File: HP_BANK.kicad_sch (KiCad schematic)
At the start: 1 part, among them J7 Conn_02x70_Odd_Even

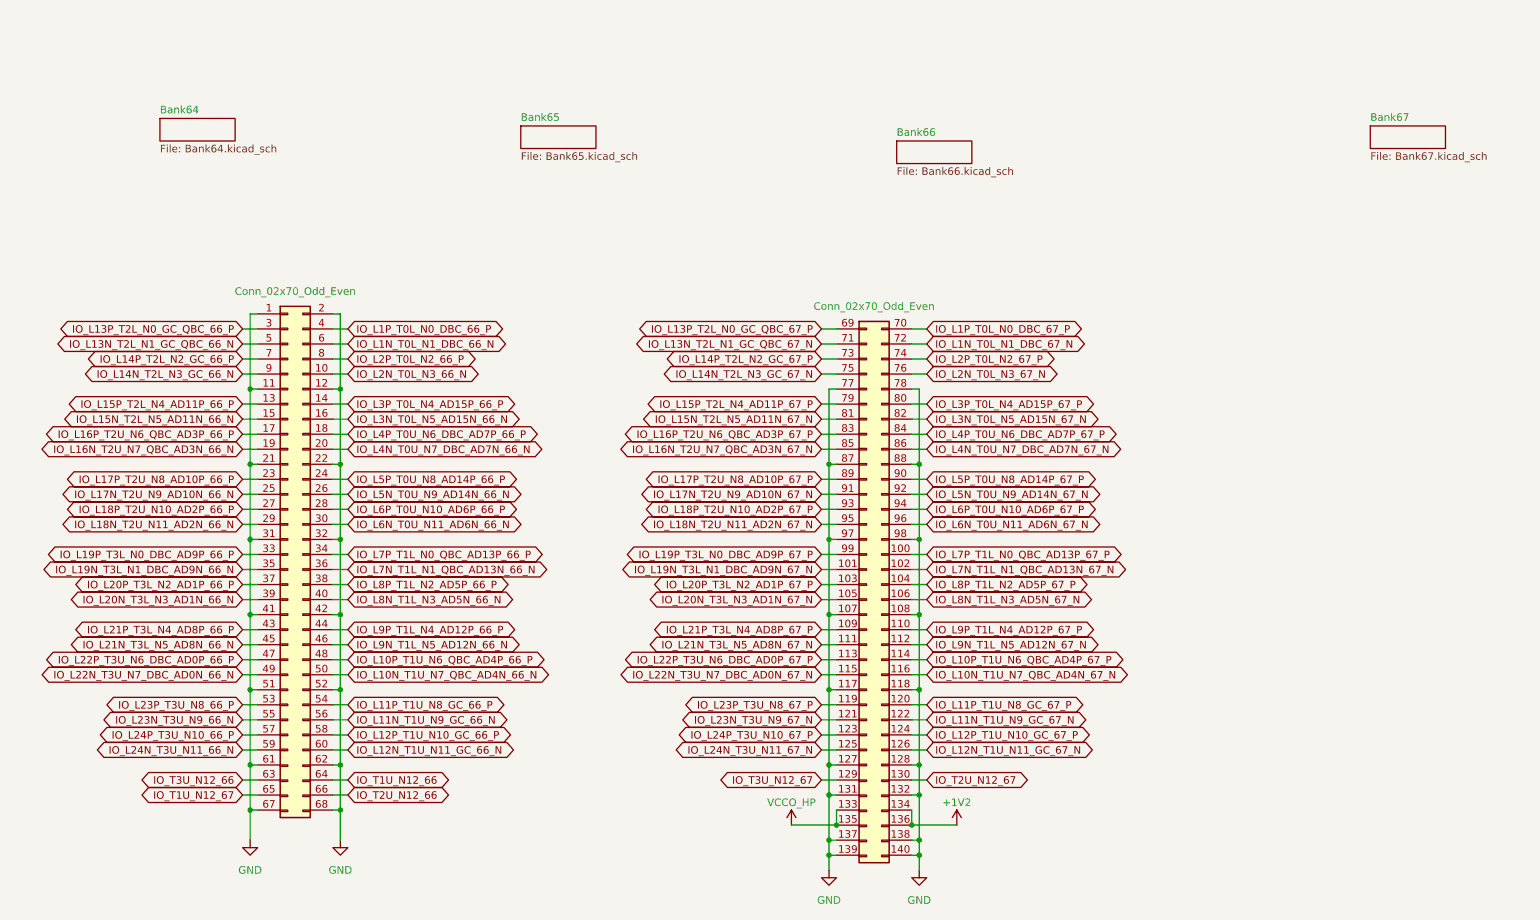
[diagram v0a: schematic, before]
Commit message: pushing the schematics works
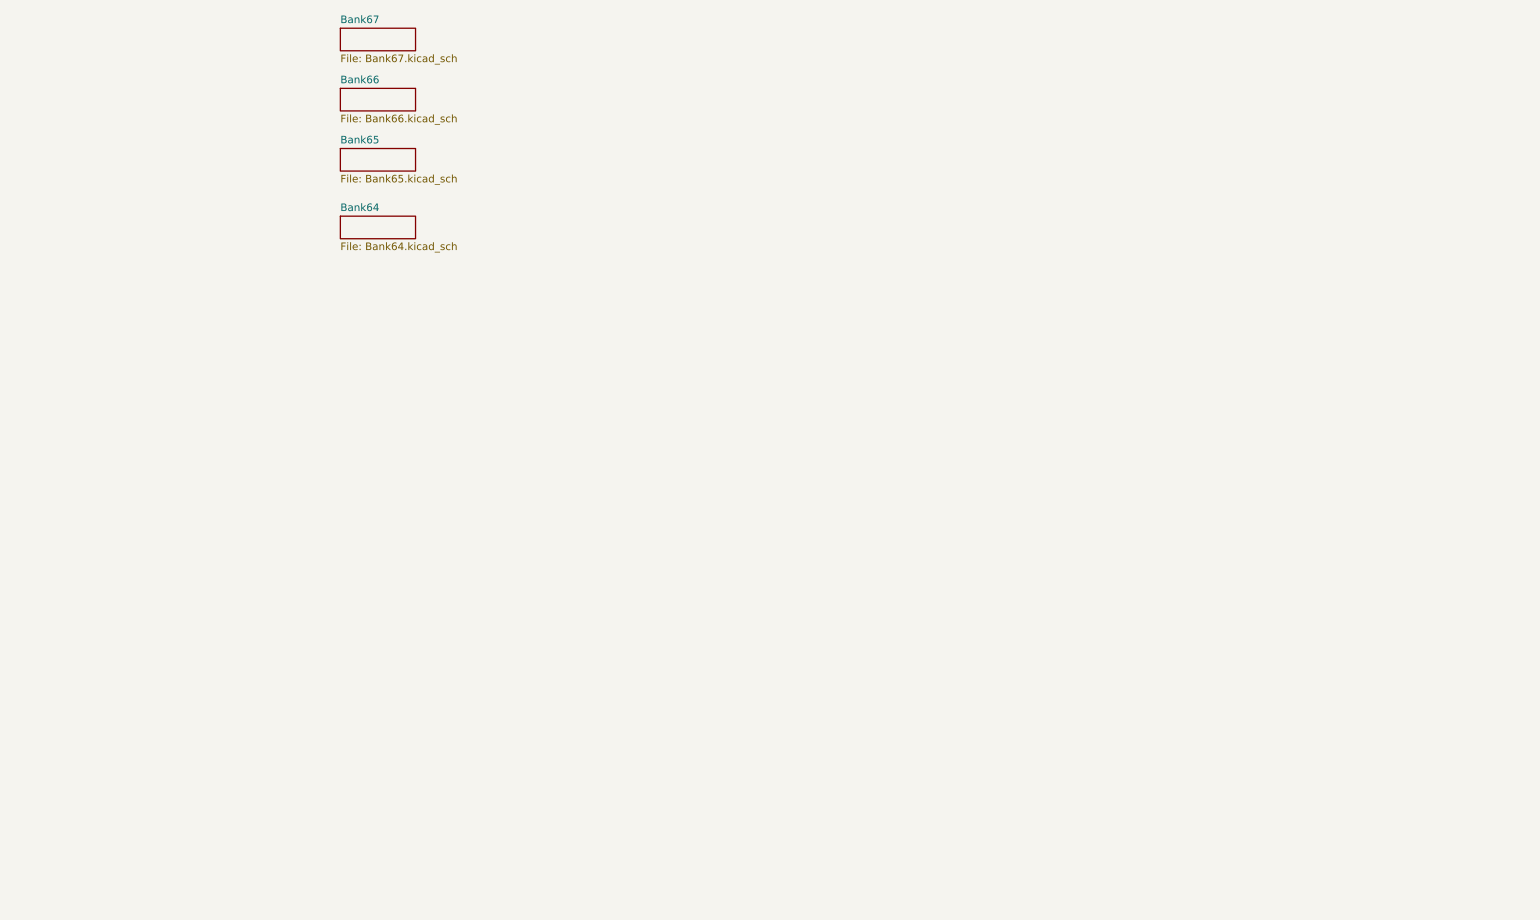
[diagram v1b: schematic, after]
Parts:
- removed J7: Conn_02x70_Odd_Even, Connector_Hirose_FX8:Hirose_FX8-140P-SV_2x70_P0.6mm, symbol dfdtc_Connector:Conn_02x70_Odd_Even
